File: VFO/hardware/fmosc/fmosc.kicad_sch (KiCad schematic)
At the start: 12 parts, among them J1 JST PH

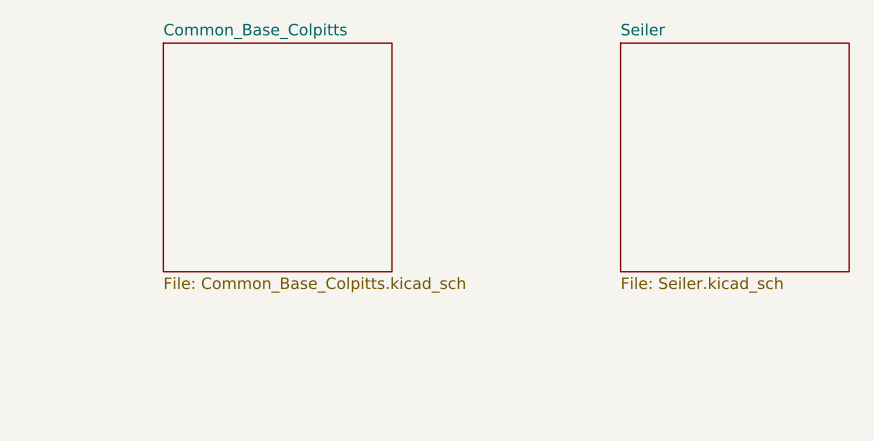
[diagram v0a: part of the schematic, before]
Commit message: release PBA-0000-0101
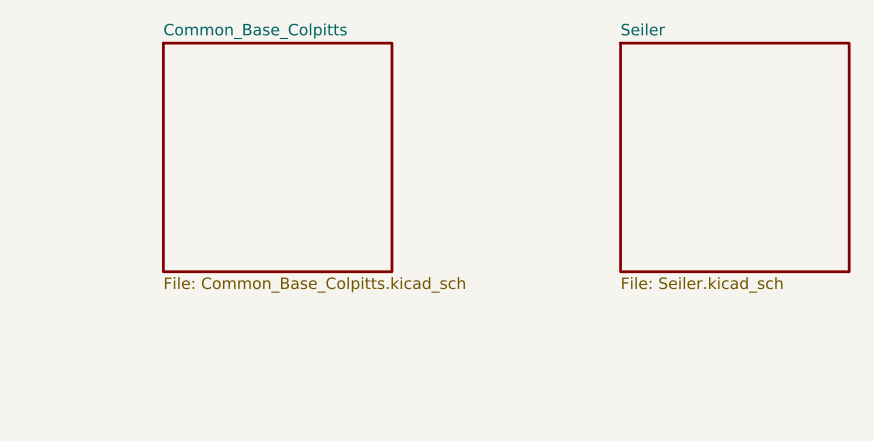
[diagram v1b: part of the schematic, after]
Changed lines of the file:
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@@
 		)
 		(instances
-			(project ""
+			(project "fmosc"
 				(path "/3dada041-f728-4295-8fb8-7b5173e4bef2"
 					(reference "#FLG01")
@@
 		)
 		(instances
-			(project ""
+			(project "fmosc"
 				(path "/3dada041-f728-4295-8fb8-7b5173e4bef2"
 					(reference "#FLG02")
@@
 		)
 		(instances
-			(project ""
+			(project "fmosc"
 				(path "/3dada041-f728-4295-8fb8-7b5173e4bef2"
 					(reference "TP1")
@@
 		)
 		(instances
-			(project ""
+			(project "fmosc"
 				(path "/3dada041-f728-4295-8fb8-7b5173e4bef2"
 					(reference "FID1")
@@
 		)
 		(instances
-			(project ""
+			(project "fmosc"
 				(path "/3dada041-f728-4295-8fb8-7b5173e4bef2"
 					(reference "TP2")
@@
 		)
 		(instances
-			(project "test1"
+			(project "fmosc"
 				(path "/3dada041-f728-4295-8fb8-7b5173e4bef2"
 					(reference "H2")
@@
 		)
 		(instances
-			(project ""
+			(project "fmosc"
 				(path "/3dada041-f728-4295-8fb8-7b5173e4bef2"
 					(reference "H1")
@@
 		)
 		(instances
-			(project "test1"
+			(project "fmosc"
 				(path "/3dada041-f728-4295-8fb8-7b5173e4bef2"
 					(reference "H3")
@@
 		)
 		(instances
-			(project "test1"
+			(project "fmosc"
 				(path "/3dada041-f728-4295-8fb8-7b5173e4bef2"
 					(reference "#PWR02")
@@
 		)
 		(instances
-			(project "test1"
+			(project "fmosc"
 				(path "/3dada041-f728-4295-8fb8-7b5173e4bef2"
 					(reference "#PWR021")
@@
 		)
 		(instances
-			(project "test1"
+			(project "fmosc"
 				(path "/3dada041-f728-4295-8fb8-7b5173e4bef2"
 					(reference "FID2")
@@
 		)
 		(instances
-			(project ""
+			(project "fmosc"
 				(path "/3dada041-f728-4295-8fb8-7b5173e4bef2"
 					(reference "D1")
@@
 		)
 		(instances
-			(project ""
+			(project "fmosc"
 				(path "/3dada041-f728-4295-8fb8-7b5173e4bef2"
 					(reference "R2")
@@
 		)
 		(instances
-			(project "test1"
+			(project "fmosc"
 				(path "/3dada041-f728-4295-8fb8-7b5173e4bef2"
 					(reference "FID3")
@@
 		)
 		(instances
-			(project ""
+			(project "fmosc"
 				(path "/3dada041-f728-4295-8fb8-7b5173e4bef2"
 					(reference "J1")
@@
 		)
 		(instances
-			(project "test1"
+			(project "fmosc"
 				(path "/3dada041-f728-4295-8fb8-7b5173e4bef2"
 					(reference "H4")
@@
 		)
 		(instances
-			(project ""
+			(project "fmosc"
 				(path "/3dada041-f728-4295-8fb8-7b5173e4bef2"
 					(reference "#PWR03")
@@
 		)
 		(instances
-			(project ""
+			(project "fmosc"
 				(path "/3dada041-f728-4295-8fb8-7b5173e4bef2"
 					(reference "#PWR01")
@@
 		(fields_autoplaced yes)
 		(stroke
-			(width 0.1524)
+			(width 0.3048)
 			(type solid)
 		)
 		(fill
-			(color 0 0 0 0.0000)
+			(color 0 255 0 1.0000)
 		)
 		(property "Sheetname" "Common_Base_Colpitts"
@@
 		(fields_autoplaced yes)
 		(stroke
-			(width 0.1524)
+			(width 0.3048)
 			(type solid)
 		)
 		(fill
-			(color 0 0 0 0.0000)
+			(color 0 255 0 1.0000)
 		)
 		(property "Sheetname" "Seiler"
